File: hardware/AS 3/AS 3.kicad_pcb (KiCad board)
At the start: 4 copper layers, 45 x 95 mm, 12 parts, among them J1 Conn_02x03_Odd_Even, J3 Connector, USB-TYPE-C-16P, U1 ESP32-S3-WROOM-1

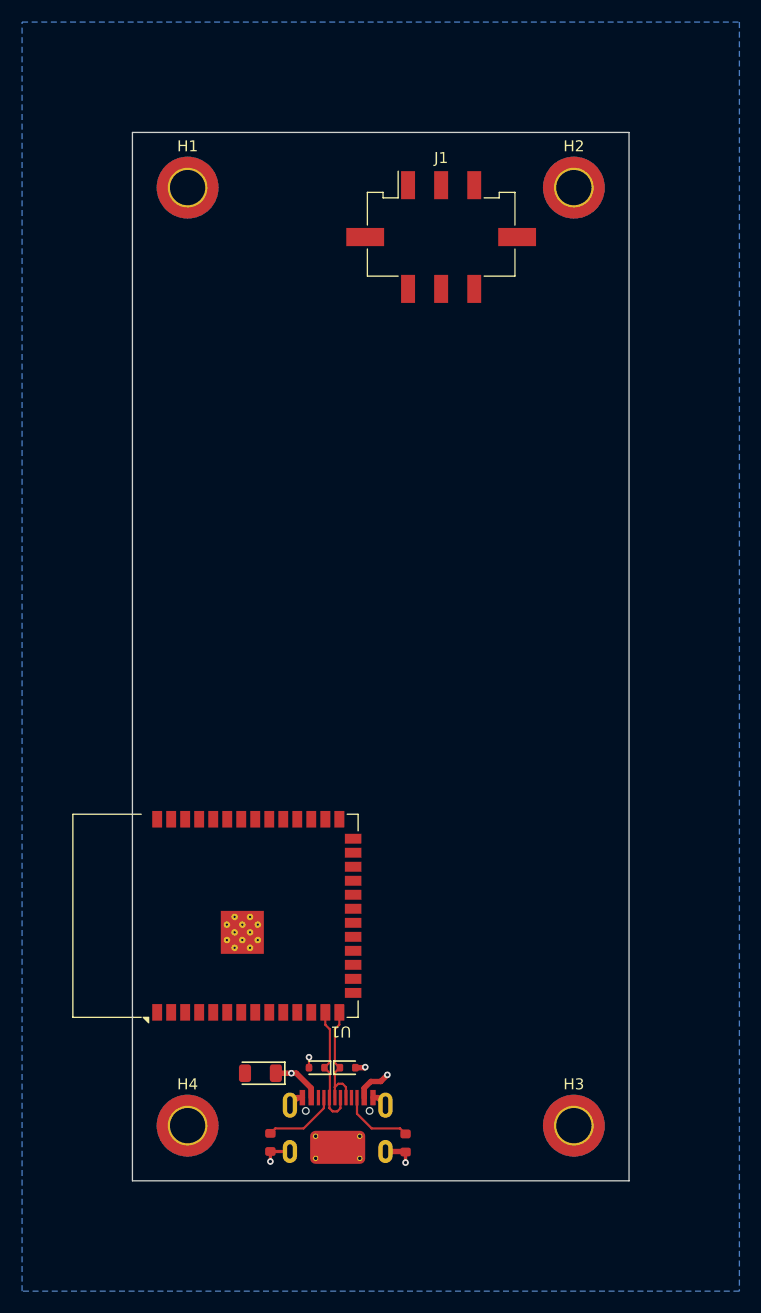
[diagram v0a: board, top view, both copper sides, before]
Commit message: PCB done????
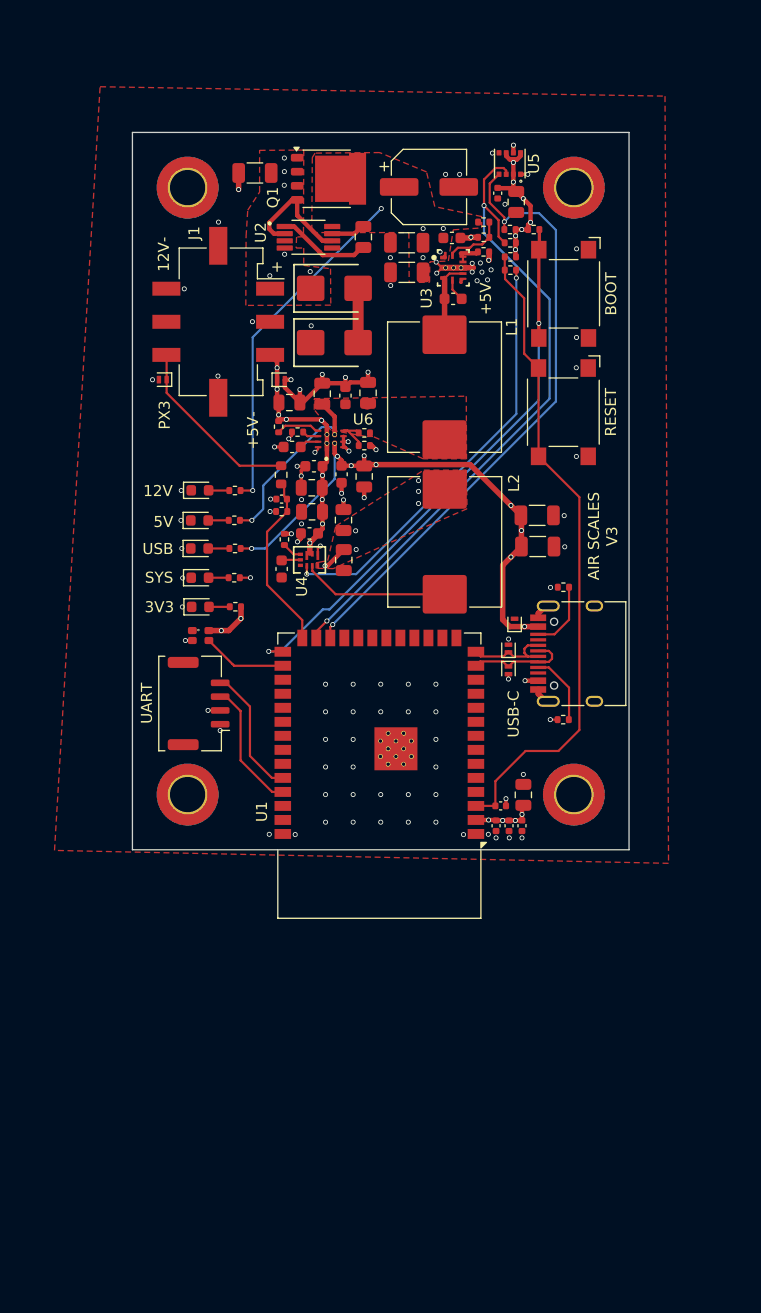
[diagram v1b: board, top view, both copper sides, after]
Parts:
- added BOOT: SW_Push, Button_Switch_SMD:SW_SPST_Omron_B3FS-100xP, F.Cu at (89.1, 64.6)
- added C1: 100nF, Capacitor_SMD:C_0402_1005Metric, F.Cu at (85.3, 112.8)
- added C10: 22uF, Capacitor_SMD:C_1206_3216Metric, F.Cu at (86.7, 87.5)
- added C11: 4.7uF, Capacitor_SMD:C_1206_3216Metric, F.Cu at (74.9, 60.0)
- added C12: 100nF, Capacitor_SMD:C_0603_1608Metric, F.Cu at (79.0, 59.6)
- added C13: 47uF, Capacitor_SMD:CP_Elec_6.3x5.7, F.Cu at (76.9, 54.9)
- added C14: 100nF, Capacitor_SMD:C_0603_1608Metric, F.Cu at (66.0, 86.3)
- added C15: 10uF, Capacitor_SMD:C_0805_2012Metric, F.Cu at (66.3, 84.4)
- added C16: 100nF, Capacitor_SMD:C_0603_1608Metric, F.Cu at (79.1, 65.1)
- added C17: 18nF, Capacitor_SMD:C_0603_1608Metric, F.Cu at (63.5, 89.6)
- added C18: 22uF, Capacitor_SMD:C_0805_2012Metric, F.Cu at (69.2, 88.8)
- added C19: 22uF, Capacitor_SMD:C_1206_3216Metric, F.Cu at (61.1, 53.7)
- added C2: 1uF, Capacitor_SMD:C_0402_1005Metric, F.Cu at (83.4, 111.0)
- added C20: 10nF, Capacitor_SMD:C_0402_1005Metric, F.Cu at (83.0, 112.8)
- added C21: 100nF, Capacitor_SMD:C_0402_1005Metric, F.Cu at (84.1, 112.8)
- added C22: 22uF, Capacitor_SMD:C_1206_3216Metric, F.Cu at (86.7, 84.7)
- added C23: 100nF, Capacitor_SMD:C_0402_1005Metric, F.Cu at (83.1, 55.5)
- added C24: 10uF, Capacitor_SMD:C_0805_2012Metric, F.Cu at (84.8, 56.3)
- added C25: 10uF, Capacitor_SMD:C_0805_2012Metric, F.Cu at (67.2, 73.7)
- added C26: 100nF, Capacitor_SMD:C_0603_1608Metric, F.Cu at (69.3, 73.8)
- added C27: 10uF, Capacitor_SMD:C_0805_2012Metric, F.Cu at (71.0, 81.2)
- added C28: 100nF, Capacitor_SMD:C_0603_1608Metric, F.Cu at (69.0, 81.0)
- added C29: 100nF, Capacitor_SMD:C_0603_1608Metric, F.Cu at (64.5, 78.5)
- added C3: 10uF, Capacitor_SMD:C_0805_2012Metric, F.Cu at (85.4, 110.0)
- added C30: 22uF, Capacitor_SMD:C_0805_2012Metric, F.Cu at (66.2, 82.2)
- added C31: 22uF, Capacitor_SMD:C_0805_2012Metric, F.Cu at (64.2, 74.5)
- added C32: 100nF, Capacitor_SMD:C_0603_1608Metric, F.Cu at (66.5, 80.2)
- added C5: 100nF, Capacitor_SMD:C_0402_1005Metric, F.Cu at (63.5, 83.2)
- added C6: 2.2uF, Capacitor_SMD:C_0805_2012Metric, F.Cu at (70.9, 59.5)
- added C7: 22uF, Capacitor_SMD:C_0805_2012Metric, F.Cu at (71.3, 73.6)
- added C8: 22uF, Capacitor_SMD:C_0805_2012Metric, F.Cu at (69.1, 85.1)
- added C9: 22uF, Capacitor_SMD:C_1206_3216Metric, F.Cu at (74.9, 62.7)
- added D10: D_TVS_Small, Diode_SMD:D_SOD-882, F.Cu at (84.1, 96.8)
- added D11: D_TVS_Small, Diode_SMD:D_SOD-882, F.Cu at (84.6, 94.4)
- added D2_1: SMBJ28A, PCM_JLCPCB:D_SMB, F.Cu at (68.3, 64.1)
- added D2_2: SMBJ14A, PCM_JLCPCB:D_SMB, F.Cu at (68.3, 69.0)
- added D4: Green, LED_SMD:LED_0603_1608Metric, F.Cu at (56.1, 85.2)
- added D5: Green, LED_SMD:LED_0603_1608Metric, F.Cu at (56.1, 82.4)
- added D6: Green, LED_SMD:LED_0603_1608Metric, F.Cu at (56.1, 90.3)
- added D7: Green, LED_SMD:LED_0603_1608Metric, F.Cu at (56.2, 93.0)
- added D8: D_TVS_Small, Diode_SMD:D_SOD-882, F.Cu at (52.8, 72.4)
- added D9: WS2812B, PCM_JLCPCB:LED-SMD_4P-L1.6-W1.5_XL-1615RGBC-WS2812B, F.Cu at (56.2, 95.6)
- added L1: 10uH, Inductor_SMD:L_Chilisin_BMRF00101040, F.Cu at (78.3, 73.1)
- added L2: 2.2uH, Inductor_SMD:L_Chilisin_BMRF00101040, F.Cu at (78.3, 87.1)
- added Q1: PSMN5R2-60YL, Package_TO_SOT_SMD:LFPAK56, F.Cu at (67.6, 54.2)
- added R1: 100K, Resistor_SMD:R_0402_1005Metric, F.Cu at (86.4, 58.8)
- added R10: 86.6kΩ, Resistor_SMD:R_0402_1005Metric, F.Cu at (65.0, 77.2)
- added R11: 1K, Resistor_SMD:R_0402_1005Metric, F.Cu at (59.3, 87.7)
- added R12: 10K, Resistor_SMD:R_0402_1005Metric, F.Cu at (71.0, 77.2)
- added R13: 4,7K, Resistor_SMD:R_0402_1005Metric, F.Cu at (71.0, 78.4)
- added R14: 86.6kΩ, Resistor_SMD:R_0402_1005Metric, F.Cu at (81.8, 60.8)
- added R15: 100K, Resistor_SMD:R_0402_1005Metric, F.Cu at (81.8, 58.1)
- added R16: 16K, Resistor_SMD:R_0402_1005Metric, F.Cu at (81.8, 59.5)
- added R17: 4.7K, Resistor_SMD:R_0402_1005Metric, F.Cu at (84.2, 60.0)
- added R18: 100K, Resistor_SMD:R_0402_1005Metric, F.Cu at (84.2, 61.3)
- added R19: 61.9K, Resistor_SMD:R_0402_1005Metric, F.Cu at (63.8, 86.9)
- added R2: 1K, Resistor_SMD:R_0402_1005Metric, F.Cu at (59.2, 85.2)
- added R20: 220, Resistor_SMD:R_0402_1005Metric, F.Cu at (59.3, 93.0)
- added R21: 1K, Resistor_SMD:R_0402_1005Metric, F.Cu at (59.2, 90.3)
- added R22: 10K, Resistor_SMD:R_0402_1005Metric, F.Cu at (63.2, 76.7)
- added R5: 4.7K, Resistor_SMD:R_0402_1005Metric, F.Cu at (59.3, 82.5)
- added R6: 4.7K, Resistor_SMD:R_0402_1005Metric, F.Cu at (84.2, 58.8)
- added R7: 10K, Resistor_SMD:R_0402_1005Metric, F.Cu at (84.2, 62.5)
- added R8: 1K, Resistor_SMD:R_0603_1608Metric, F.Cu at (63.5, 81.0)
- added R9: 2K, Resistor_SMD:R_0402_1005Metric, F.Cu at (63.5, 84.3)
- added RESET: SW_Push, Button_Switch_SMD:SW_SPST_Omron_B3FS-100xP, F.Cu at (89.0, 75.3)
- added U2: LM74610QDGKTQ1, LM74610QDGKTQ1:SOP65P490X110-8N, F.Cu at (66.0, 59.5)
- added U3: LMR604205SRAKRQ1, LMR60420:RAK0009A-MFG, F.Cu at (79.1, 62.3)
- added U4: TPS62901RPJR, TPS62901:QFN_902RPJR_TEX, F.Cu at (66.0, 88.7)
- added U5: BME280, BME280:PSON65P250X250X100-8N, F.Cu at (84.2, 52.8)
- added U6: TPS2121RUXR, TPS2121RUXR:IC_TPS2121RUXR, F.Cu at (68.0, 77.8)
- added UART: Conn_01x04, Connector_Molex:Molex_CLIK-Mate_502382-0470_1x04-1MP_P1.25mm_Vertical, F.Cu at (56.0, 101.8)
- D1: value ESD321DYAR -> Green; footprint PCM_JLCPCB:D_SOD-523 -> LED_SMD:LED_0603_1608Metric
- D2: value ESD321DYAR -> D_TVS_Small; footprint PCM_JLCPCB:D_SOD-523 -> Diode_SMD:D_SOD-882
- D3: value ESD441DPLR -> D_TVS_Small; footprint PCM_JLCPCB:D_SOD-123FL -> Diode_SMD:D_SOD-882
- R3, R4: footprint PCM_JLCPCB:R_0603 -> Resistor_SMD:R_0402_1005Metric
- USB-C: renamed from J3; value Connector, USB-TYPE-C-16P -> USB_C_Receptacle_USB2.0_16P; footprint PCM_JLCPCB:TYPE-C-SMD_HX-TYPE-C-16PIN -> Connector_USB:USB_C_Receptacle_HRO_TYPE-C-31-M-12
- moved D2 62.6 mm to (63.5, 72.4)
- moved R3 52.4 mm to (89.1, 91.2), turned to 180 degrees
- moved D1 48.2 mm to (56.1, 87.7), turned to 0 degrees
- moved USB-C 48.2 mm to (90.8, 97.2), turned to 90 degrees
- moved R4 46.6 mm to (89.0, 103.2), turned to 180 degrees
- moved D3 42.9 mm to (84.1, 98.7), turned to -90 degrees
- moved H3 30.0 mm to (90.0, 110.0)
- moved H4 30.0 mm to (55.0, 110.0)
- moved J1 21.6 mm to (57.8, 67.2), turned to -90 degrees
- moved U1 19.5 mm to (72.4, 108.3), turned to 180 degrees
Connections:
- D1 pad 1: /D- -> GND
- D1 pad 2: GND -> Net-(D1-A)
- D2 pad 1: /D+ -> +5VMUX
- D3 pad 1: VBUS -> /D-
- J1 pad 3: unconnected-(J1-Pin_3-Pad3) -> +5VMUX
- J1 pad 4: /PX3_Signal -> GND
- J1 pad 5: +5V -> unconnected-(J1-Pin_5-Pad5)
- J1 pad 6: GND -> /PX3_Signal
- J1 pad MP: (no net) -> GND
- U1 pad 2: VDD33 -> +3.3V
- U1 pad 26: unconnected-(U1-IO45-Pad26) -> /PX3_PRESS
- U1 pad 28: unconnected-(U1-IO35-Pad28) -> /LED
- U1 pad 34: /PX3_PRESS -> unconnected-(U1-IO41-Pad34)
- U1 pad 5: /LED -> unconnected-(U1-IO5-Pad5)
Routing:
- net /SDA: track 0.00 -> 59.7 mm, vias 0 -> 2
- net /EN: track 0.00 -> 59.2 mm
- net /SCL: track 0.00 -> 57.0 mm, vias 0 -> 2
- net /BOOT: track 0.00 -> 52.0 mm, vias 0 -> 2
- net +5VBus: track 0.00 -> 50.3 mm, vias 0 -> 10
- net /PG: track 0.00 -> 38.9 mm, vias 0 -> 2
- net GND: track 10.2 -> 42.4 mm, vias 4 -> 101
- net +12VA: track 0.00 -> 31.6 mm, vias 0 -> 6
- net +3.3V: track 0.00 -> 28.1 mm, vias 0 -> 20
- net +5VMUX: track 0.00 -> 23.9 mm, vias 0 -> 10
- net +5V: track 0.00 -> 16.9 mm, vias 0 -> 1
- net /PX3_Signal: track 0.00 -> 16.6 mm
- net /PX3_PRESS: track 0.00 -> 16.3 mm
- net Net-(U4-SW): track 0.00 -> 13.3 mm
- net /TXD0: track 0.00 -> 11.9 mm
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- added copper zone on F.Cu, net +12V
- added copper zone on In2.Cu, net +12V
- added copper zone on F.Cu, net +12VA
- added copper zone on In2.Cu, net +12VA
- added copper zone on F.Cu, net +3.3V
- added copper zone on In2.Cu, net +3.3V
- added copper zone on F.Cu, net +5V
- added copper zone on In2.Cu, net +5VBus
- added copper zone on In2.Cu, net +5VMUX
- added copper zone on F.Cu, net GND
- added copper zone on In1.Cu, net GND
- removed copper zone on B.Cu, net GND
- removed copper zone on In2.Cu, net VBUS
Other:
- board size 45 x 95 mm -> 45 x 65 mm
- board text added: "+"
- board text added: "+5V"
- board text added: "+5V-"
- board text added: "12V"
- board text added: "12V-"
- board text added: "3V3"
- board text added: "5V"
- board text added: "AIR SCALES"
- board text added: "PX3"
- board text added: "SYS"
- board text added: "USB"
- board text added: "V3"
